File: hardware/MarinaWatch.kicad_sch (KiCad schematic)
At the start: 49 parts, among them J201 USB_C_Receptacle_USB2.0_16P, J901 Screw_Terminal_01x06, J902 Screw_Terminal_01x06, SW101 SW_Push, SW102 SW_Push, U101 ESP32-S3-MINI-1, U301 LMV321, U302 LMV321, U303 LMV321, U304 ESP32-S3-WROOM-1

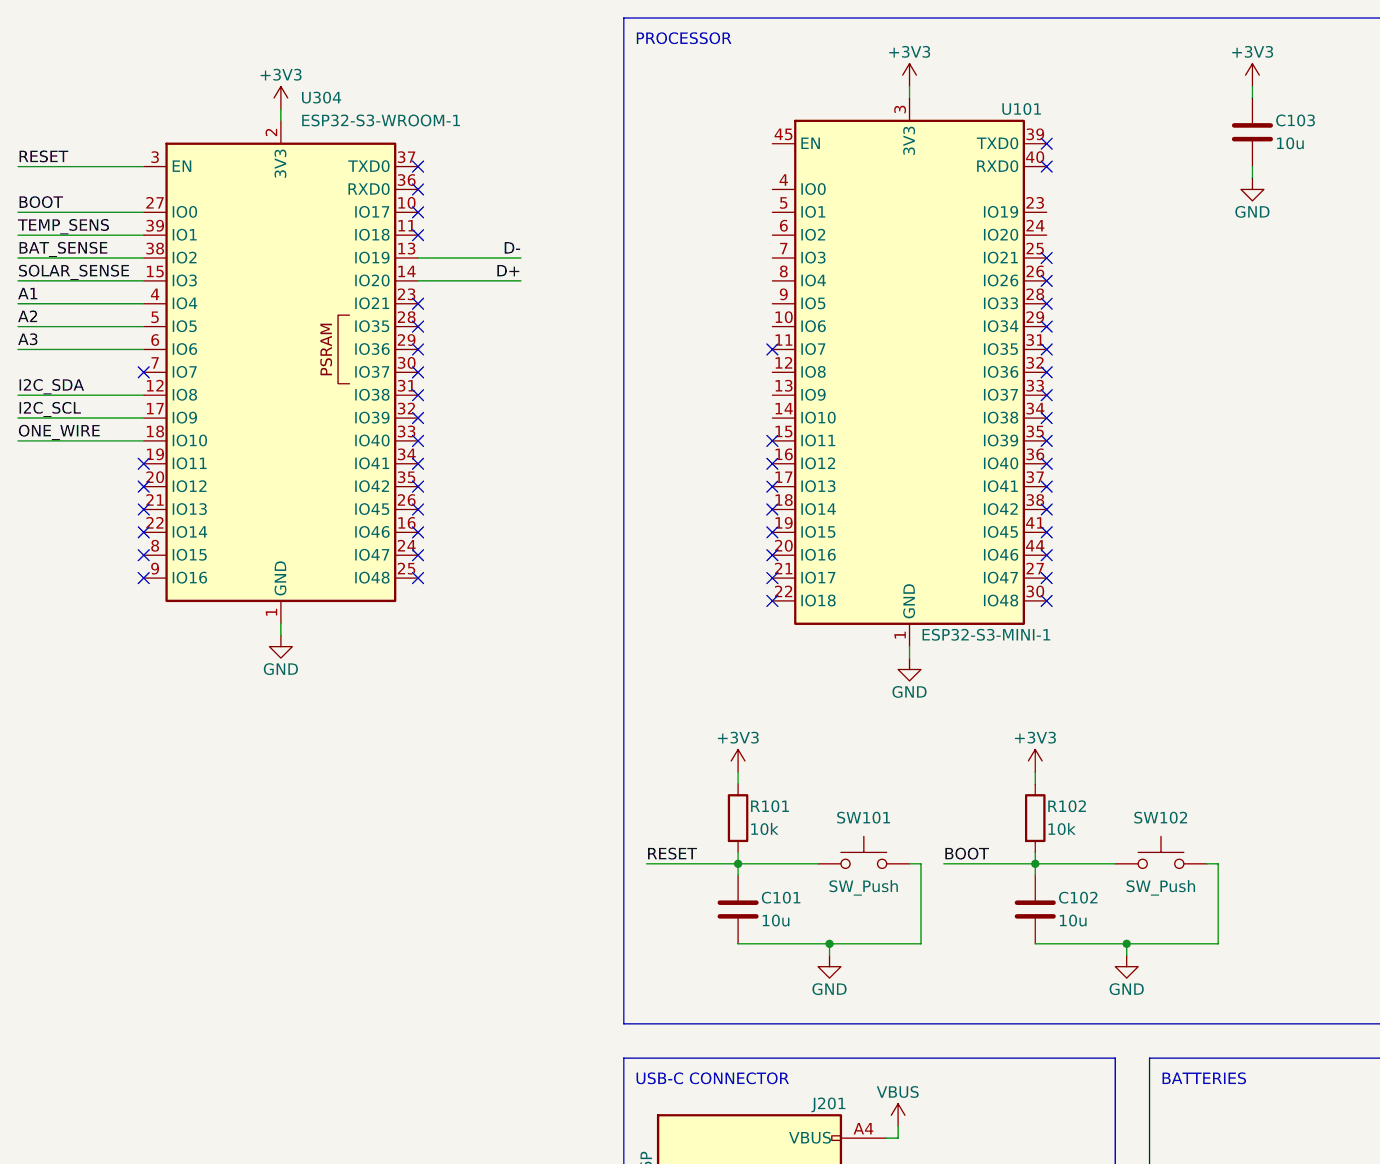
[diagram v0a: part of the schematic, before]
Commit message: Recond draft of HW
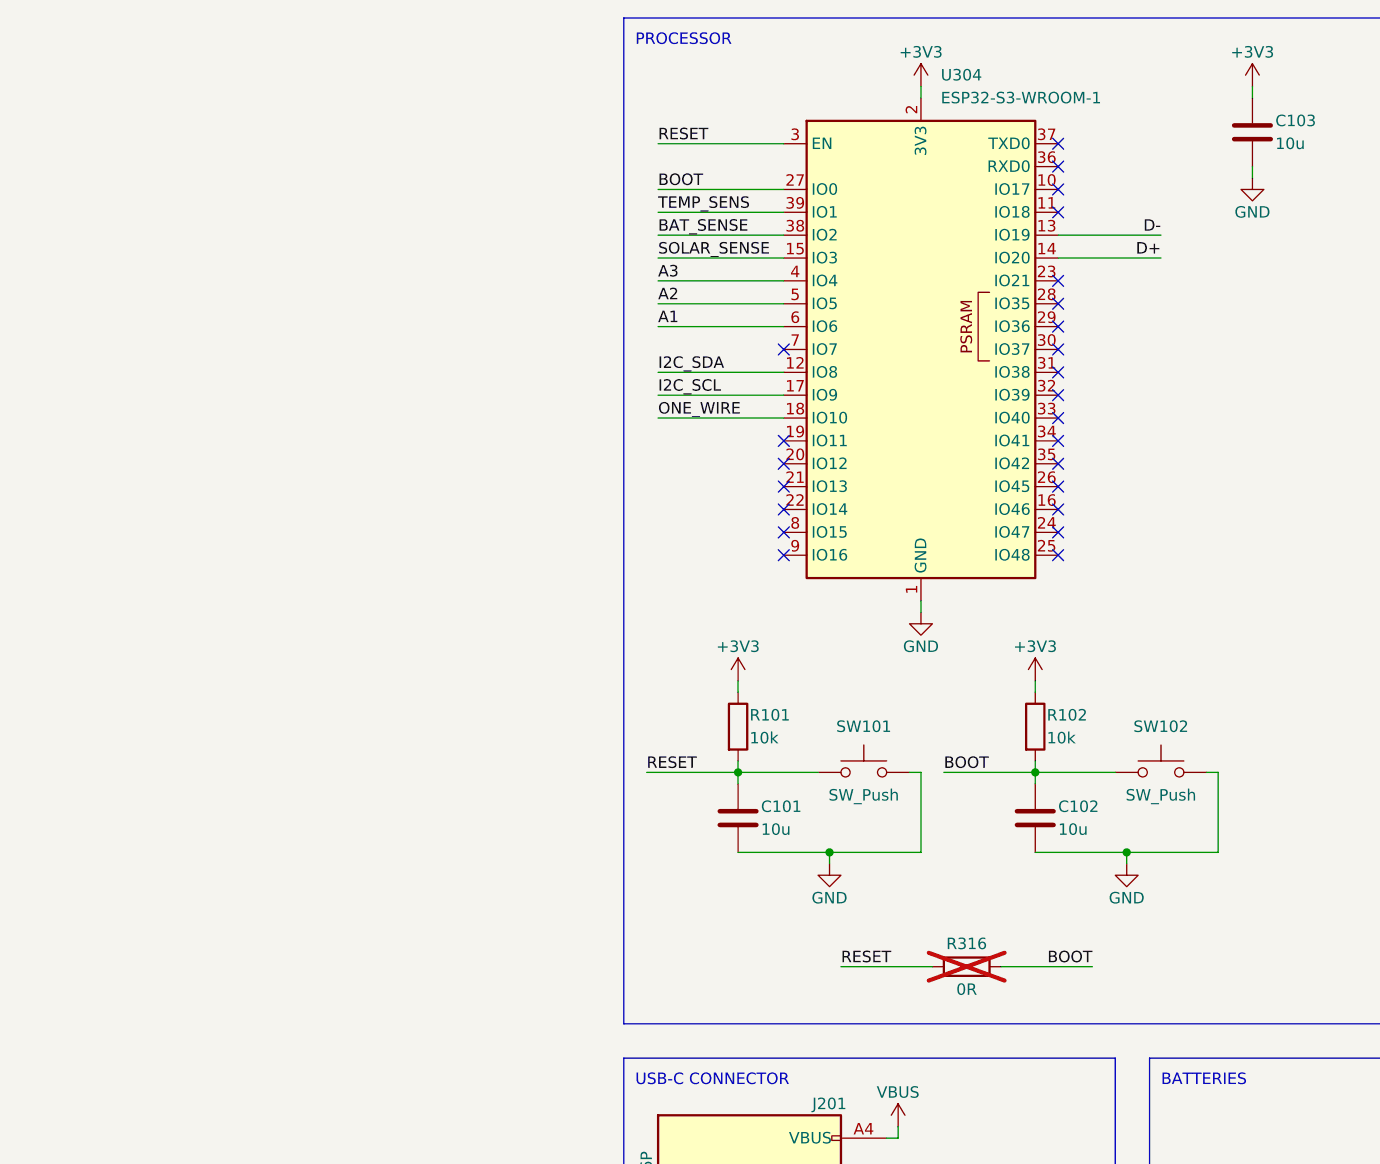
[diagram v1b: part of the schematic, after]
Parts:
- removed U101: ESP32-S3-MINI-1, RF_Module:ESP32-S2-MINI-1, symbol RF_Module:ESP32-S3-MINI-1
- added R316: 0R, Resistor_SMD:R_0603_1608Metric_Pad0.98x0.95mm_HandSolder, symbol Device:R
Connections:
- net A1: now also U304.6 (IO6); no longer U304.4 (IO4)
- net A3: now also U304.4 (IO4); no longer U304.6 (IO6)
- net BOOT: now also R316.2
- net RESET: now also R316.1
- no-connect marks 57 -> 30
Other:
- moved on the sheet: C101, C102, R101, R102, SW101, SW102, U304
